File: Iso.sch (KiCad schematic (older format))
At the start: 7 parts, among them U12 Si8421

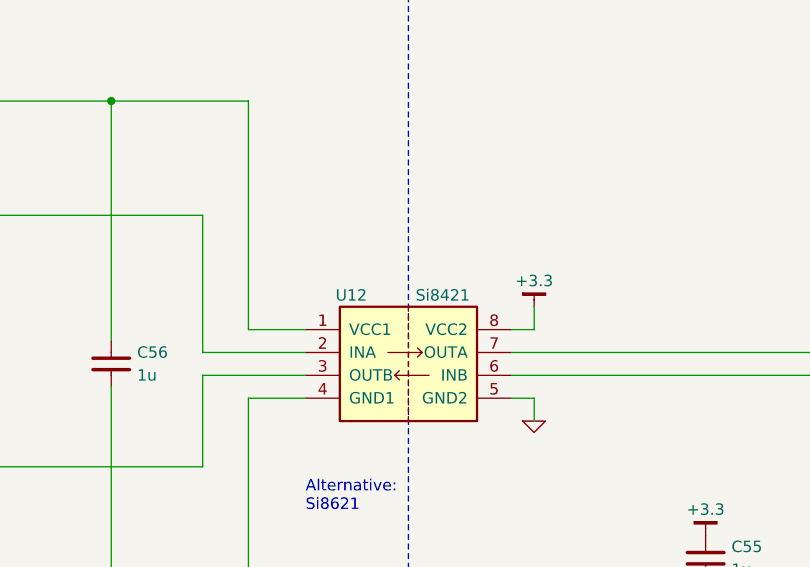
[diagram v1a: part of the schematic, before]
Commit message: Finish PCB
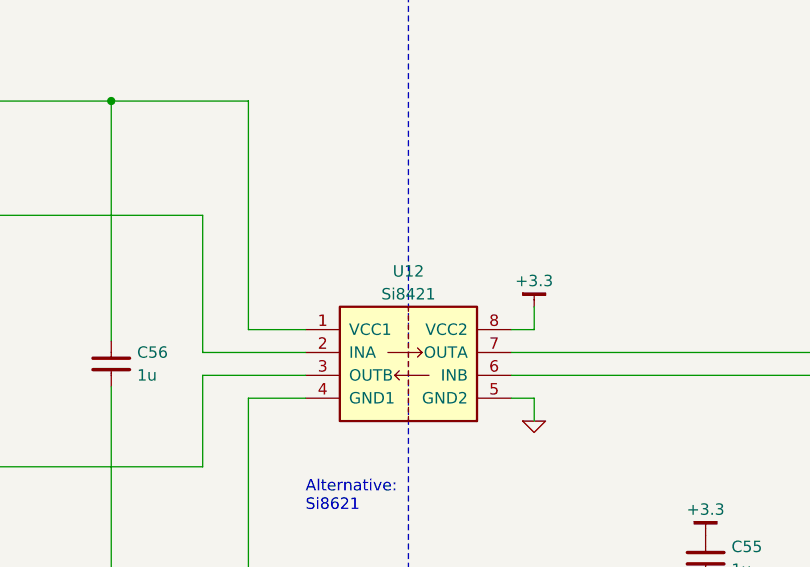
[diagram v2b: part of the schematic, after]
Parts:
- removed C54, C57: 220p, IPC7351-Nominal:CAPC1608X55, symbol C-0603
- removed R40, R51: 100, IPC7351-Nominal:RESC1608X50, symbol R-0603
- added C54, C57: 220p, IPC7351-Nominal:CAPC1005X55, symbol C-0402
- added R40, R51: 100, IPC7351-Nominal:RESC1005X40, symbol R-0402
- U12: BOM (none) -> DIST DIGIKEY 336-1755-5-ND
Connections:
- net ISO_GND: now also C54.1, C57.1
- net ISO_IN: now also R51.2
- net ISO_OUT: now also C57.2, R40.2
- net at U12.2 (INA): now also C54.2, R51.1
- net at U12.3 (OUTB): now also R40.1
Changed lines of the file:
@@
 $EndComp
 $Comp
-L GND #PWR0112
+L GND #PWR098
 U 1 1 55D17F73
 P 8200 4750
-F 0 "#PWR0112" H 8200 4750 30  0001 C CNN
+F 0 "#PWR098" H 8200 4750 30  0001 C CNN
 F 1 "GND" H 8200 4680 30  0001 C CNN
 F 2 "" H 8200 4750 60  0000 C CNN
@@
 Text HLabel 2200 3100 0    50   Input ~ 0
 ISO_IN
-$Comp
-L R-0603 R51
-U 1 1 55D56AFF
-P 3800 3100
-F 0 "R51" V 3612 3100 50  0000 C CNN
-F 1 "100" V 3712 3100 50  0000 C CNN
-F 2 "IPC7351-Nominal:RESC1608X50" H 3800 3100 50  0001 C CNN
-F 3 "" H 3800 3150 60  0000 C CNN
-F 4 "RES SMD 100 1% [0603]" H 4550 3650 60  0001 C CNN "BOM"
-F 5 "Value" H 3800 3100 60  0001 C CNN "Manuf"
-	1    3800 3100
-	0    1    1    0
-$EndComp
 Text HLabel 2200 4200 0    50   Output ~ 0
 ISO_OUT
@@
 	3900 3100 6000 3100
 $Comp
-L +3.3 #PWR0113
+L +3.3 #PWR099
 U 1 1 55D5749C
 P 8200 4500
-F 0 "#PWR0113" H 8200 4550 30  0001 C CNN
+F 0 "#PWR099" H 8200 4550 30  0001 C CNN
 F 1 "+3.3" H 8200 4613 50  0000 C CNN
 F 2 "" H 8200 4500 60  0000 C CNN
@@
 U 1 1 55D574BC
 P 6900 3750
-F 0 "U12" H 6650 4050 50  0000 C CNN
-F 1 "Si8421" H 7050 4050 50  0000 C CNN
+F 0 "U12" H 6900 4155 50  0000 C CNN
+F 1 "Si8421" H 6900 4055 50  0000 C CNN
 F 2 "IPC7351-Nominal:SOIC127P600X175-8" H 6900 3750 50  0001 C CNN
 F 3 "" H 6900 3750 60  0000 C CNN
+F 4 "DIST DIGIKEY 336-1755-5-ND" H 6900 3750 60  0001 C CNN "BOM"
 	1    6900 3750
 	1    0    0    -1
@@
 	6200 3900 6200 4900
 $Comp
-L +3.3 #PWR0114
+L +3.3 #PWR0100
 U 1 1 55D575AD
 P 7450 3500
-F 0 "#PWR0114" H 7450 3550 30  0001 C CNN
+F 0 "#PWR0100" H 7450 3550 30  0001 C CNN
 F 1 "+3.3" H 7450 3613 50  0000 C CNN
 F 2 "" H 7450 3500 60  0000 C CNN
@@
 	7450 3600 7450 3500
 $Comp
-L GND #PWR0115
+L GND #PWR0101
 U 1 1 55D57601
 P 7450 4000
-F 0 "#PWR0115" H 7450 4000 30  0001 C CNN
+F 0 "#PWR0101" H 7450 4000 30  0001 C CNN
 F 1 "GND" H 7450 3930 30  0001 C CNN
 F 2 "" H 7450 4000 60  0000 C CNN
@@
 Wire Wire Line
 	3700 3100 2200 3100
-$Comp
-L R-0603 R40
-U 1 1 55DBC1C9
-P 5000 4200
-F 0 "R40" V 4812 4200 50  0000 C CNN
-F 1 "100" V 4912 4200 50  0000 C CNN
-F 2 "IPC7351-Nominal:RESC1608X50" H 5000 4200 50  0001 C CNN
-F 3 "" H 5000 4250 60  0000 C CNN
-F 4 "RES SMD 100 1% [0603]" H 5750 4750 60  0001 C CNN "BOM"
-F 5 "Value" H 5000 4200 60  0001 C CNN "Manuf"
-	1    5000 4200
-	0    1    1    0
-$EndComp
 Wire Wire Line
 	2200 4200 4900 4200
-$Comp
-L C-0603 C?
-U 1 1 55DBCD14
-P 4200 3550
-AR Path="/55C7FF09/55DBCD14" Ref="C?"  Part="1"
-AR Path="/55D119A9/55DBCD14" Ref="C54"  Part="1"
-F 0 "C54" H 4087 3500 50  0000 R CNN
-F 1 "220p" H 4087 3600 50  0000 R CNN
-F 2 "IPC7351-Nominal:CAPC1608X55" H 4200 3550 50  0001 C CNN
-F 3 "" H 4190 3525 60  0000 C CNN
-F 4 "CAP MLCC 220p C0G 50V 10% [0603]" H 5000 4100 60  0001 C CNN "BOM"
-F 5 "Value" H 4200 3550 60  0001 C CNN "Manuf"
-	1    4200 3550
-	-1   0    0    1
-$EndComp
 Wire Wire Line
 	4200 3450 4200 3100
@@
 	4200 3650 4200 4900
 Connection ~ 4200 4900
-$Comp
-L C-0603 C?
-U 1 1 55DBCDBA
-P 4600 4550
-AR Path="/55C7FF09/55DBCDBA" Ref="C?"  Part="1"
-AR Path="/55D119A9/55DBCDBA" Ref="C57"  Part="1"
-F 0 "C57" H 4487 4500 50  0000 R CNN
-F 1 "220p" H 4487 4600 50  0000 R CNN
-F 2 "IPC7351-Nominal:CAPC1608X55" H 4600 4550 50  0001 C CNN
-F 3 "" H 4590 4525 60  0000 C CNN
-F 4 "CAP MLCC 220p C0G 50V 10% [0603]" H 5400 5100 60  0001 C CNN "BOM"
-F 5 "Value" H 4600 4550 60  0001 C CNN "Manuf"
-	1    4600 4550
-	-1   0    0    1
-$EndComp
 Wire Wire Line
 	4600 4450 4600 4200
@@
 	4600 4650 4600 4900
 Connection ~ 4600 4900
+$Comp
+L R-0402 R51
+U 1 1 5600C06F
+P 3800 3100
+F 0 "R51" V 3612 3100 50  0000 C CNN
+F 1 "100" V 3712 3100 50  0000 C CNN
+F 2 "IPC7351-Nominal:RESC1005X40" H 3800 3100 50  0001 C CNN
+F 3 "" H 3800 3150 60  0000 C CNN
+F 4 "RES SMD 100 1% [0402]" H 4550 3650 60  0001 C CNN "BOM"
+	1    3800 3100
+	0    1    1    0
+$EndComp
+$Comp
+L C-0402 C?
+U 1 1 5600C8E4
+P 4200 3550
+AR Path="/55C7FF09/5600C8E4" Ref="C?"  Part="1"
+AR Path="/55C7F4BB/5600C8E4" Ref="C?"  Part="1"
+AR Path="/55D119A9/5600C8E4" Ref="C54"  Part="1"
+F 0 "C54" H 4087 3500 50  0000 R CNN
+F 1 "220p" H 4087 3600 50  0000 R CNN
+F 2 "IPC7351-Nominal:CAPC1005X55" H 4200 3550 50  0001 C CNN
+F 3 "" H 4190 3525 60  0000 C CNN
+F 4 "CAP MLCC 220p C0G 50V 10% [0402]" H 5000 4100 60  0001 C CNN "BOM"
+	1    4200 3550
+	-1   0    0    1
+$EndComp
+$Comp
+L C-0402 C?
+U 1 1 5600CF4E
+P 4600 4550
+AR Path="/55C7FF09/5600CF4E" Ref="C?"  Part="1"
+AR Path="/55C7F4BB/5600CF4E" Ref="C?"  Part="1"
+AR Path="/55D119A9/5600CF4E" Ref="C57"  Part="1"
+F 0 "C57" H 4487 4500 50  0000 R CNN
+F 1 "220p" H 4487 4600 50  0000 R CNN
+F 2 "IPC7351-Nominal:CAPC1005X55" H 4600 4550 50  0001 C CNN
+F 3 "" H 4590 4525 60  0000 C CNN
+F 4 "CAP MLCC 220p C0G 50V 10% [0402]" H 5400 5100 60  0001 C CNN "BOM"
+	1    4600 4550
+	-1   0    0    1
+$EndComp
+$Comp
+L R-0402 R40
+U 1 1 5600D582
+P 5000 4200
+F 0 "R40" V 4812 4200 50  0000 C CNN
+F 1 "100" V 4912 4200 50  0000 C CNN
+F 2 "IPC7351-Nominal:RESC1005X40" H 5000 4200 50  0001 C CNN
+F 3 "" H 5000 4250 60  0000 C CNN
+F 4 "RES SMD 100 1% [0402]" H 5750 4750 60  0001 C CNN "BOM"
+	1    5000 4200
+	0    1    1    0
+$EndComp
 $EndSCHEMATC
